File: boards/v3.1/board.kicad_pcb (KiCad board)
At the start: 2 copper layers, 113.3 x 98 mm, 66 parts, among them J1 KF301-2P, J2 KF301-2P, J3 KF301-2P, J4 KF301-2P, J5 KF301-2P, J6 KF301-2P, P1 Pin Header, P2 Pin Header, P3 Pin Header, P4 Pin Header, P5 Pin Header, SW1 SS-12D00G 4mm, SW2 SS-12D00G 4mm, T1 ZMPT101B, T2 ZMPT101B, T3 ZMPT101B, U1 TL082, U2 TL082, U3 TL082, U4 TL082, U5 TL082, U6 TL082

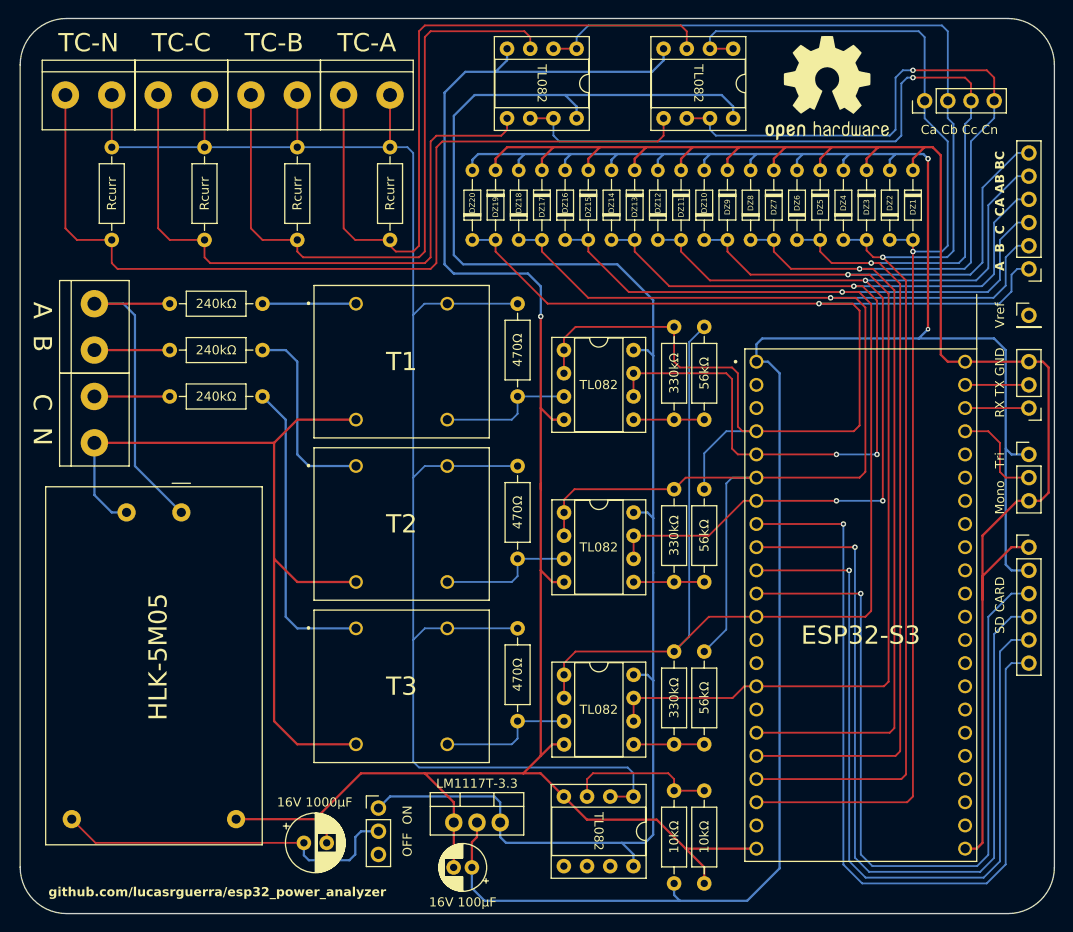
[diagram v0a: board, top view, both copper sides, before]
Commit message: Update firmware and boards
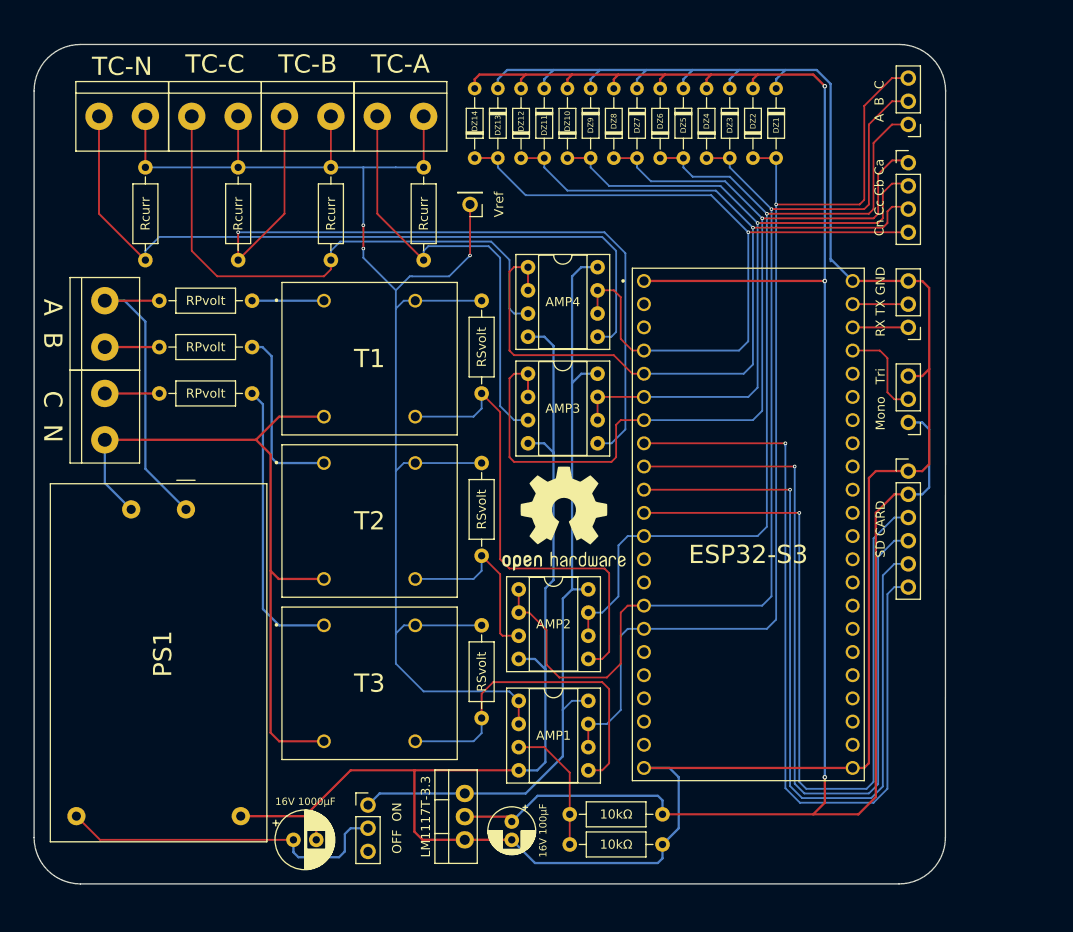
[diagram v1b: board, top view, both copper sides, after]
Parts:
- removed DZ15, DZ16, DZ17, DZ18, DZ19, DZ20: 3.3V, Diode_THT:D_DO-34_SOD68_P7.62mm_Horizontal
- removed R13: 330kΩ, Resistor_THT:R_Axial_DIN0207_L6.3mm_D2.5mm_P10.16mm_Horizontal
- removed R14: 56kΩ, Resistor_THT:R_Axial_DIN0207_L6.3mm_D2.5mm_P10.16mm_Horizontal
- removed R15, R16, R17, R18: Rcurr, Resistor_THT:R_Axial_DIN0207_L6.3mm_D2.5mm_P10.16mm_Horizontal
- removed U1, U2, U3, U4, U5, U6: TL082, Package_DIP:DIP-8_W7.62mm_Socket
- added AMP1: TL082, Package_DIP:DIP-8_W7.62mm_Socket, F.Cu at (146.8, 110.8)
- added AMP2: TL082, Package_DIP:DIP-8_W7.62mm_Socket, F.Cu at (146.8, 98.6)
- added AMP3: TL082, Package_DIP:DIP-8_W7.62mm_Socket, F.Cu at (147.8, 75.0)
- added AMP4: TL082, Package_DIP:DIP-8_W7.62mm_Socket, F.Cu at (147.8, 63.3)
- P4: footprint Connector_PinHeader_2.54mm:PinHeader_1x06_P2.54mm_Vertical -> Connector_PinHeader_2.54mm:PinHeader_1x03_P2.54mm_Vertical
- R10, R12: value 56kΩ -> Rcurr
- R11, R9: value 330kΩ -> Rcurr
- R3, R4, R5: value 240kΩ -> RPvolt
- R6, R7, R8: value 470Ω -> RSvolt
- moved R12 66.2 mm to (105.9, 62.5), turned to 90 degrees
- moved P2 62.4 mm to (141.5, 56.4), turned to 180 degrees
- moved G*** 55.3 mm to (151.8, 90.9)
- moved R10 51.6 mm to (116.1, 62.5), turned to 90 degrees
- moved R11 45.2 mm to (126.2, 62.5), turned to 90 degrees
- moved R9 28.4 mm to (136.4, 62.5), turned to 90 degrees
- moved P4 20.6 mm to (189.5, 47.7)
- moved DZ10 17.5 mm to (152.1, 51.4)
- moved DZ11 17.5 mm to (149.6, 43.7)
- moved DZ3 17.5 mm to (169.9, 43.7)
- moved DZ4 17.5 mm to (167.4, 51.4)
- moved DZ7 17.5 mm to (159.8, 43.7)
- moved DZ14 17.5 mm to (142.0, 51.4)
- moved DZ1 17.5 mm to (175.0, 43.7)
- moved DZ12 17.5 mm to (147.1, 51.4)
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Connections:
- net Net-(U1A-+) renamed V1.65
- DZ1 pad 2: Current A -> Treated Wave C
- DZ10 pad 1: Treated Wave BC -> Current B
- DZ11 pad 2: Treated Wave AB -> Current C
- DZ12 pad 1: Treated Wave AB -> Current C
- DZ13 pad 2: Treated Wave CA -> Current N
- DZ14 pad 1: Treated Wave CA -> Current N
- DZ2 pad 1: Current A -> Treated Wave C
- DZ3 pad 2: Current B -> Treated Wave B
- DZ4 pad 1: Current B -> Treated Wave B
- DZ5 pad 2: Current C -> Treated Wave A
- DZ6 pad 1: Current C -> Treated Wave A
- DZ7 pad 2: Current N -> Current A
- DZ8 pad 1: Current N -> Current A
- DZ9 pad 2: Treated Wave BC -> Current B
- MCU1 pad J1_12: Treated Wave C -> Treated Wave A
- MCU1 pad J1_15: Treated Wave BC -> Treated Wave B
- MCU1 pad J1_16: unconnected-(MCU1-GPIO10-PadJ1_16) -> Treated Wave C
- MCU1 pad J1_17: Current N -> unconnected-(MCU1-GPIO11-PadJ1_17)
- MCU1 pad J1_18: Current C -> unconnected-(MCU1-GPIO12-PadJ1_18)
- MCU1 pad J1_19: Current B -> unconnected-(MCU1-GPIO13-PadJ1_19)
- MCU1 pad J1_20: Current A -> unconnected-(MCU1-GPIO14-PadJ1_20)
- MCU1 pad J1_4: Treated Wave A -> Current N
- MCU1 pad J1_5: Treated Wave CA -> Current C
- MCU1 pad J1_6: Treated Wave B -> Current B
- MCU1 pad J1_7: Treated Wave AB -> Current A
- R10 pad 1: Treated Wave C -> TC B-1
- R10 pad 2: Net-(U2B-+) -> TC A-2
- R11 pad 1: Treated Wave B -> TC C-1
- R11 pad 2: Net-(U3B-+) -> TC A-2
- R12 pad 1: Treated Wave A -> TC N-1
- R12 pad 2: Net-(U3B-+) -> TC A-2
- R9 pad 1: Treated Wave A -> TC A-1
- R9 pad 2: Net-(U2B-+) -> TC A-2
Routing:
- net Treated Wave BC: track 127.2 -> 0.00 mm, vias 1 -> 0
- net Treated Wave CA: track 113.2 -> 0.00 mm, vias 3 -> 0
- net Treated Wave AB: track 108.4 -> 0.00 mm, vias 3 -> 0
- net Vin: track 179.7 -> 88.0 mm
- net Current B: track 157.7 -> 82.8 mm
- net GND: track 385.7 -> 314.1 mm, vias 1 -> 0
- net Current N: track 157.7 -> 88.3 mm, vias 2 -> 1
- net Current C: track 168.0 -> 104.4 mm, vias 2 -> 1
- net Treated Wave C: track 173.7 -> 112.2 mm
- net Treated Wave A: track 142.6 -> 102.2 mm
- net Wave A: track 14.9 -> 52.1 mm
- net TC A-1: track 79.8 -> 47.9 mm
- net Current A: track 136.8 -> 107.5 mm
- net Treated Wave B: track 146.9 -> 119.8 mm
- net Wave C: track 15.0 -> 37.5 mm
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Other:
- board size 113.3 x 98 mm -> 99.8 x 91.9 mm
- board text removed: "github.com/lucasrguerra/esp32_power_analyzer"
